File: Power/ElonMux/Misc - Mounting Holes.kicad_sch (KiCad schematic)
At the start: 18 parts

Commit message: Added MODE, U0TX, U0RX, sourced from Mouser
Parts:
- C1201, C1202, C1203, C1204: Manufacturer Part Number C0603V102KDRAC7867 -> C0603C102MDRAC7081; Supplier Digikey -> Mouser Electronics; Supplier Part Number 399-12306-1-ND -> 80-C0603C102MDRAC

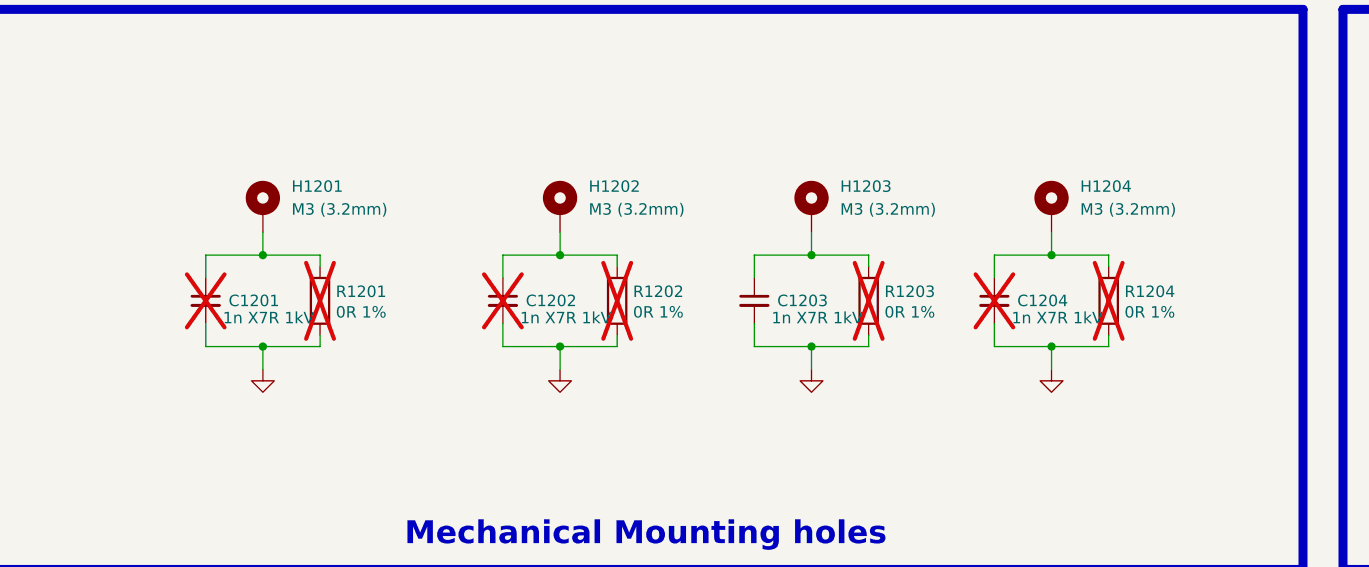
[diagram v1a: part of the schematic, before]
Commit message: Final version with Buck-Boost
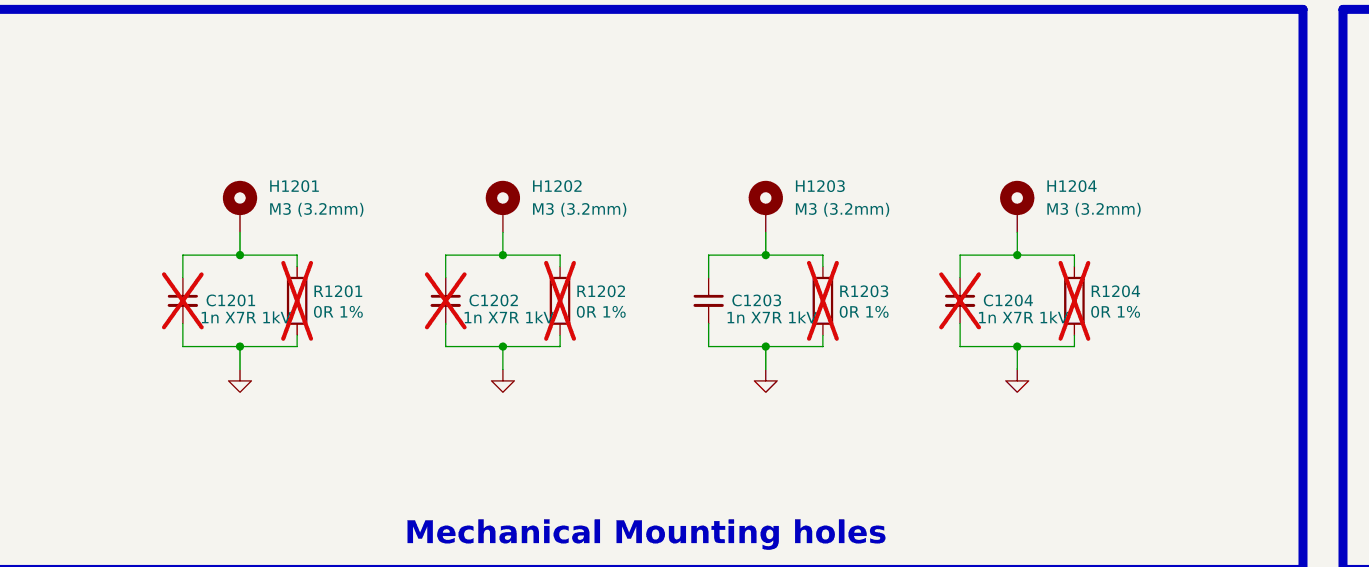
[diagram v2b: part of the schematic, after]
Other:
- moved on the sheet: C1201, C1202, C1203, C1204, H1201, H1202, H1203, H1204, R1201, R1202, R1203, R1204
